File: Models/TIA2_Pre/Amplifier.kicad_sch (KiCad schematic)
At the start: 4 parts, among them U1 AD8615

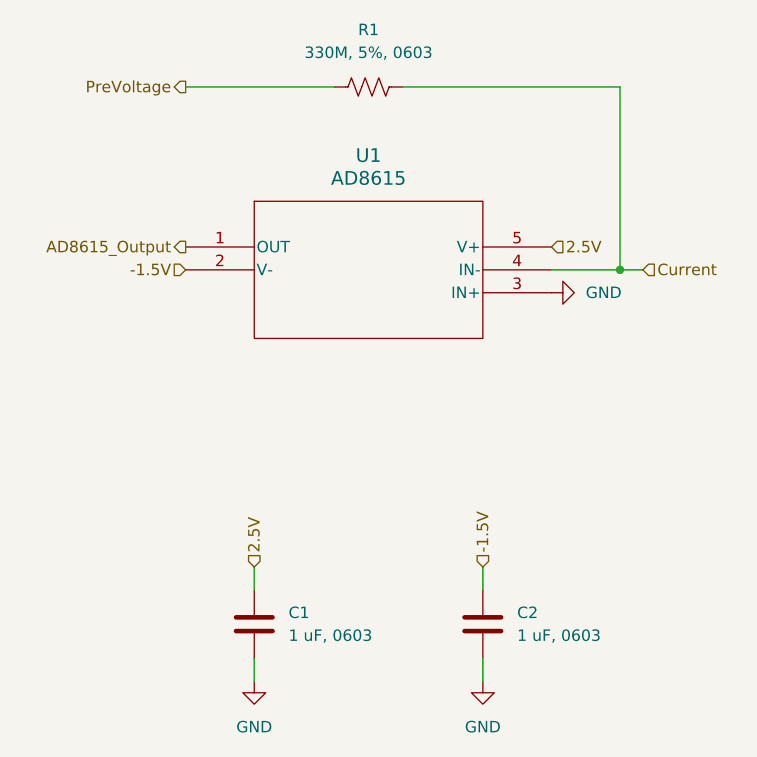
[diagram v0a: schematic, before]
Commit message: Save progress
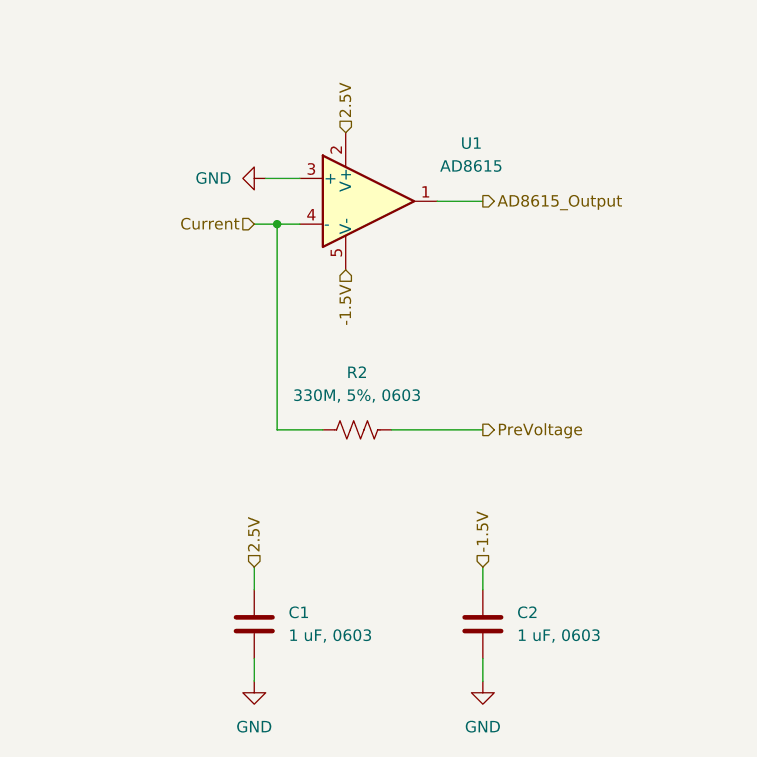
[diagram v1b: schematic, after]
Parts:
- removed R1: 330M, 5%, 0603, symbol Device:R_US
- removed U1: AD8615, symbol Vendor:AD8615
- added R2: 330M, 5%, 0603, symbol Device:R_US
- added U1: AD8615, symbol Amplifier_Operational:OP179GRT
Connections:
- net -1.5V: now also U1.5 (V-)
- net 2.5V: now also U1.2 (V+)
- net AD8615_Output: now also U1.1
- net Current: now also R2.1, U1.4 (-)
- net GND: now also U1.3 (+)
- net PreVoltage: now also R2.2
